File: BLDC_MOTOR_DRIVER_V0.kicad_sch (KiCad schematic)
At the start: 54 parts, among them J1 Conn_01x05_Pin, J10 Conn_01x01_Socket, J11 Conn_01x01_Socket, J12 Conn_01x01_Socket, J13 Conn_01x01_Socket, J14 Conn_01x01_Socket, J2 Conn_01x01_Socket, J3 Conn_01x01_Socket, J4 Conn_01x01_Socket, J5 Conn_01x01_Socket, J6 Conn_01x01_Socket, J7 Conn_01x01_Socket, J8 Conn_01x01_Socket, J9 Conn_01x01_Socket, Q1 N-MOSFET, Q2 N-MOSFET, Q3 N-MOSFET, Q4 N-MOSFET, Q5 N-MOSFET, Q6 N-MOSFET, U1 3-phase Gate Driver, U2 Micro controller, U4 3.3V Regurator, U5 FIN1019MTCX

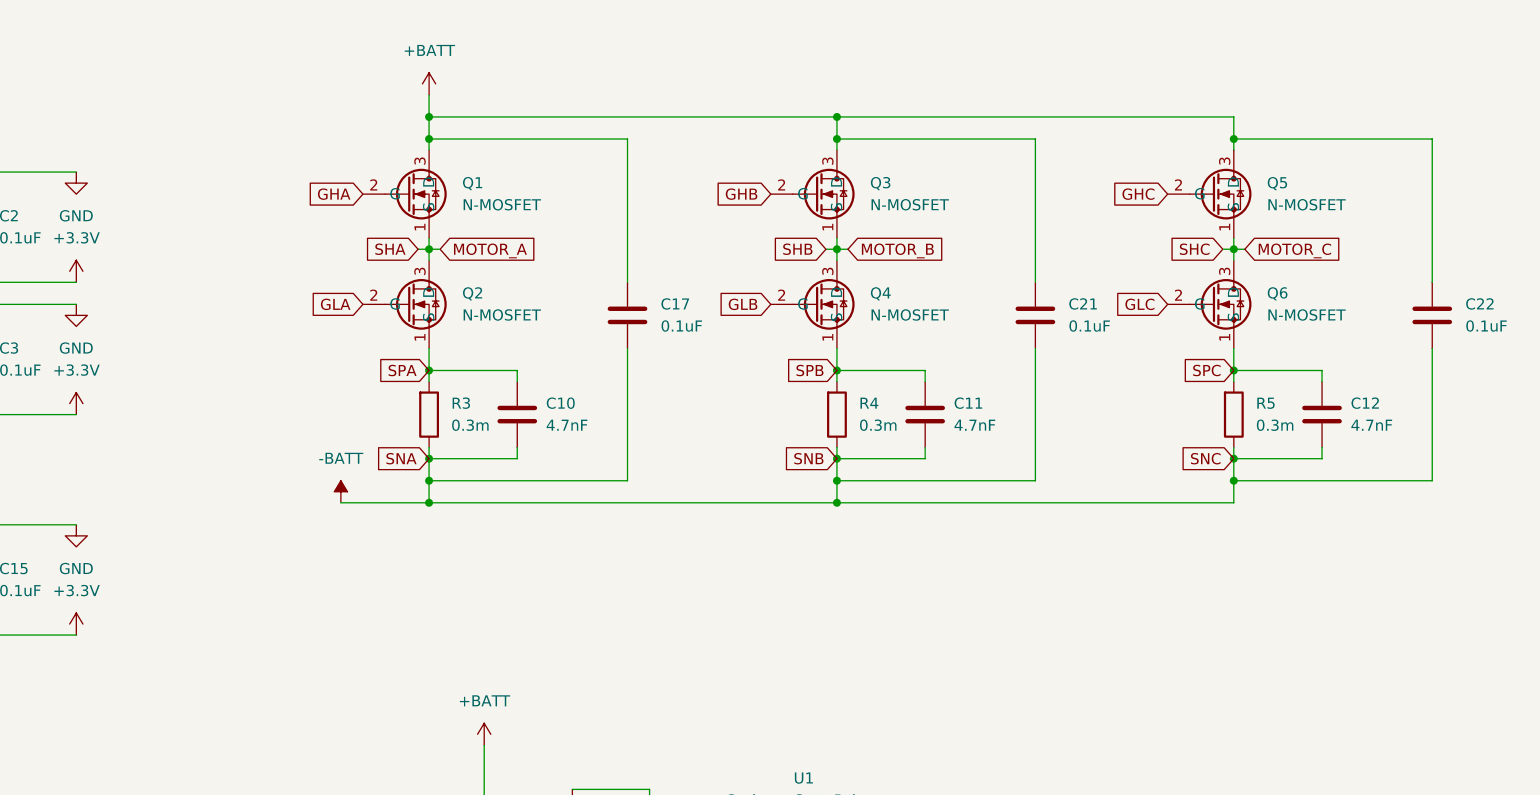
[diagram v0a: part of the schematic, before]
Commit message: dg
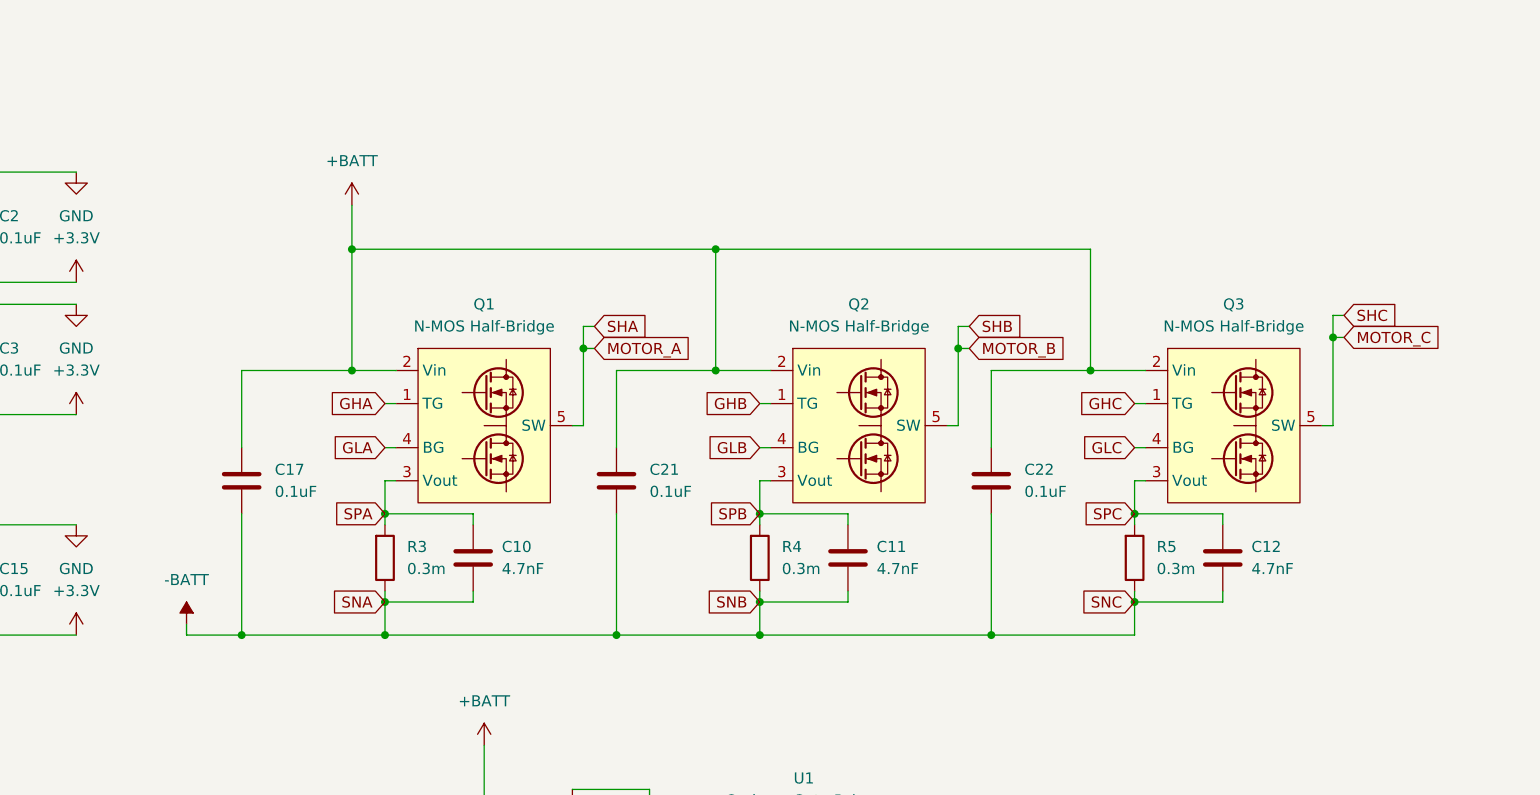
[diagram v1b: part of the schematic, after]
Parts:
- removed Q1, Q2, Q3, Q4, Q5, Q6: N-MOSFET, NTMFS5C468NLT1G:NTMFS5C468NLT1G, symbol NTMFS5C468NLT1G:NTMFS5C468NLT1G
- added Q1, Q2, Q3: N-MOS Half-Bridge, CSD87588N:CSD87588N, symbol CSD87588N:CSD87588N
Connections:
- net +BATT: now also Q1.2 (Vin), Q2.2 (Vin), Q3.2 (Vin)
- net GHA: now also Q1.1 (TG)
- net GHB: now also Q2.1 (TG)
- net GHC: now also Q3.1 (TG)
- net GLA: now also Q1.4 (BG)
- net GLB: now also Q2.4 (BG)
- net GLC: now also Q3.4 (BG)
- net MOTOR_A: now also Q1.5 (SW)
- net MOTOR_B: now also Q2.5 (SW)
- net MOTOR_C: now also Q3.5 (SW)
- net SPA: now also Q1.3 (Vout)
- net SPB: now also Q2.3 (Vout)
- net SPC: now also Q3.3 (Vout)
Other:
- moved on the sheet: C10, C11, C12, C17, C21, C22, R3, R4, R5
